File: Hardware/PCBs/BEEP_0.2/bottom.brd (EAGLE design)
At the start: 85 x 73 mm, 53 parts, among them IC1 74HCT00D, Q1 DMN2075U, Q2 IRLML2244, Q5 IRLML2244, Q6 IRLML2244, Q8 IRLML2244, U1 LM239AMDREP, U2 ATTINY10-TSHR

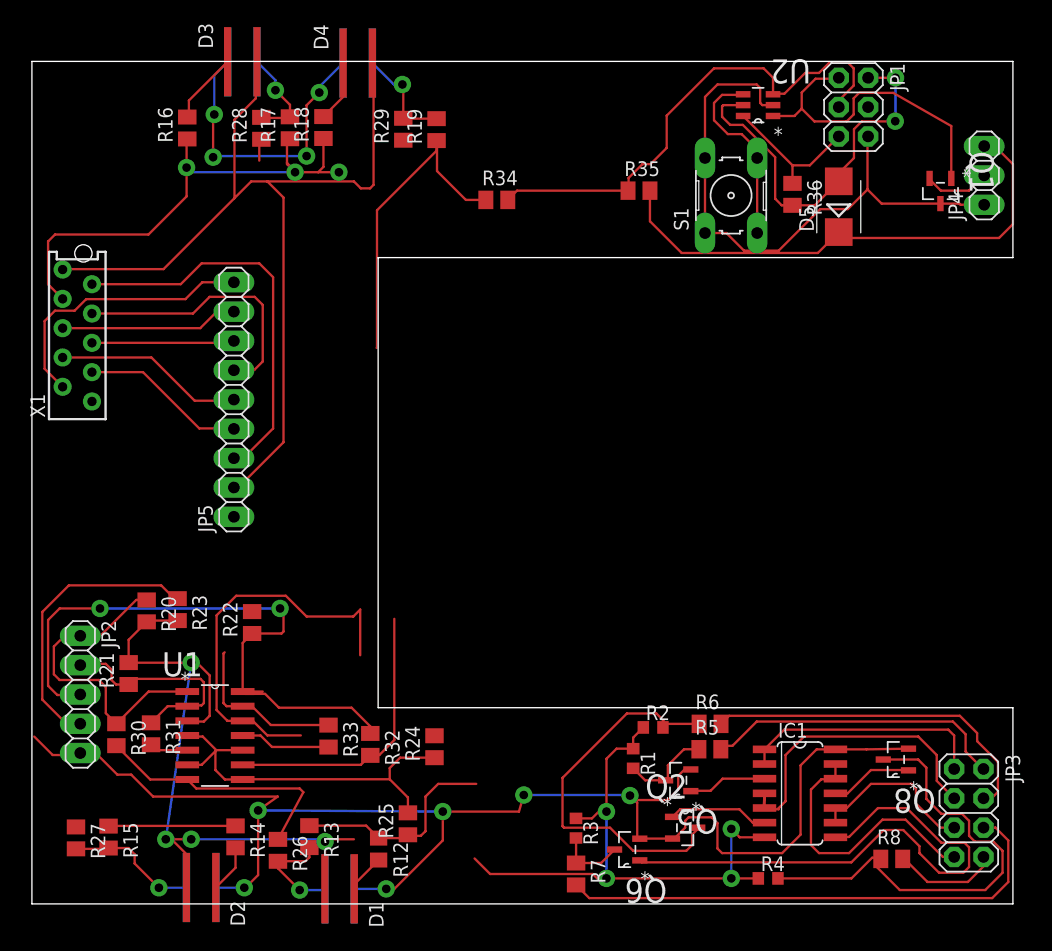
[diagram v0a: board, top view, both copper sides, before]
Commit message: continue work on bottom pcbs
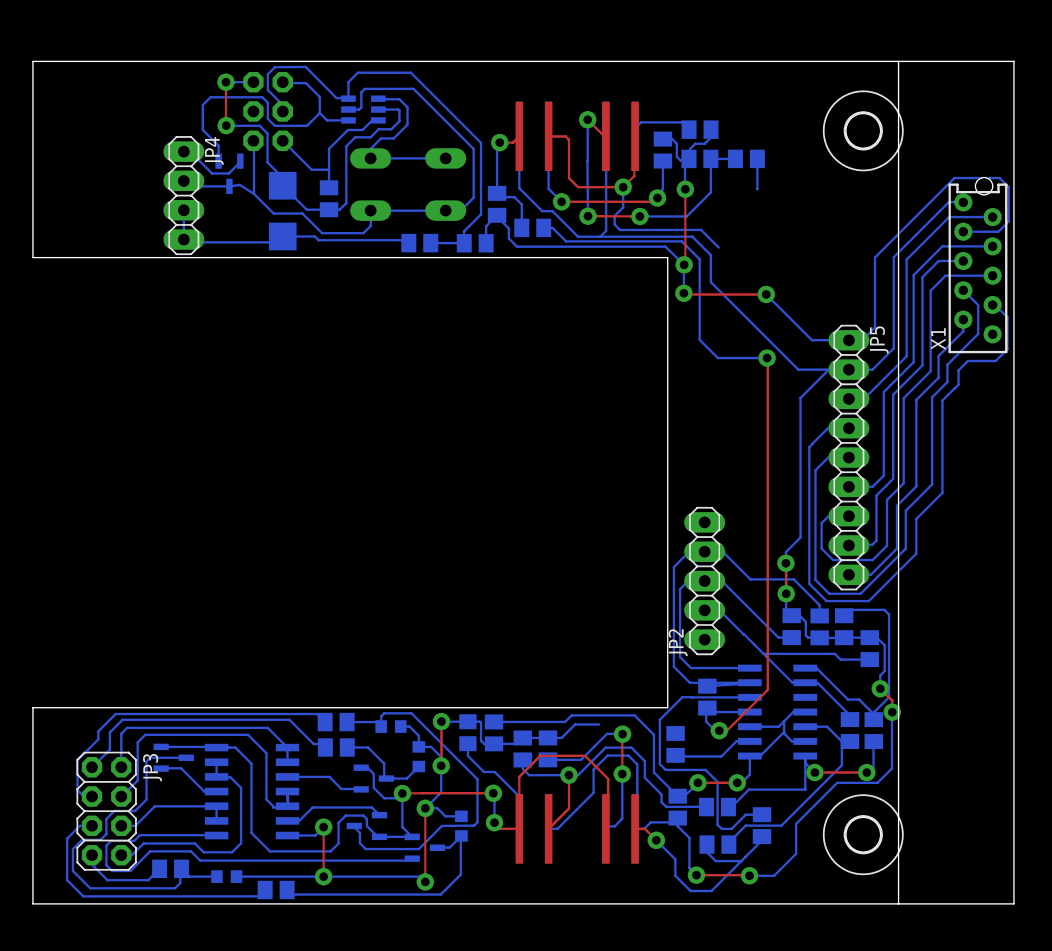
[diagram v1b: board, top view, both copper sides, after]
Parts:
- added U$1, U$2: (no value), holes:3,0
- JP4: device pinhead:1X03 -> pinhead:1X04
- moved X1 78.3 mm to (82.0, 55.1)
- moved JP3 74.7 mm to (6.48, 8.03)
- moved JP4 69.4 mm to (13.2, 61.4), turned to 270 degrees
- moved R30 65.6 mm to (72.9, 15.0), flipped to the bottom
- moved R21 64.3 mm to (72.6, 22.1), flipped to the bottom
- moved Q8 62.6 mm to (12.3, 12.7), flipped to the bottom
- moved R8 62.5 mm to (12.0, 3.04), flipped to the bottom
- moved Q1 61.6 mm to (17.1, 63.3), flipped to the bottom
- moved R31 60.6 mm to (70.9, 15.0), flipped to the bottom
- moved R20 60.5 mm to (70.4, 24.0), flipped to the bottom
- moved R15 56.6 mm to (63.3, 6.78), flipped to the bottom
- moved R23 55.7 mm to (68.3, 24.0), flipped to the bottom
- moved R27 55.6 mm to (59.4, 5.14), flipped to the bottom, turned to 0 degrees
- moved JP2 55.0 mm to (58.3, 28.0), turned to 90 degrees
- moved JP5 53.5 mm to (70.8, 38.7), turned to 270 degrees
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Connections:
- net +7V: now also JP4.4
- net BATT_GND: now also JP4.2; no longer JP4.1
- net PWM_IN1: now also JP3.2; no longer JP3.1
- net PWM_IN2: now also JP3.4; no longer JP3.3
- net PWM_IN3: now also JP3.6; no longer JP3.5
- net PWM_IN4: now also JP3.8; no longer JP3.7
- net PWM_OUT1: now also JP3.1; no longer JP3.2
- net PWM_OUT2: now also JP3.3; no longer JP3.4
- net PWM_OUT3: now also JP3.5; no longer JP3.6
- net PWM_OUT4: now also JP3.7; no longer JP3.8
- net SWITCHED_GND: now also JP4.1; no longer JP4.2
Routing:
- net N$49: track 7.85 -> 69.1 mm, vias 0 -> 2
- net +5V: track 153.8 -> 103.0 mm, vias 10 -> 4
- net COLOR_DIODE_2: track 14.3 -> 54.5 mm
- net COLOR_DIODE_1: track 16.4 -> 48.3 mm
- net ENC_R1: track 54.3 -> 24.8 mm, vias 2 -> 0
- net COLOR_SENSOR_3: track 12.4 -> 41.0 mm
- net +3V3: track 144.8 -> 167.8 mm, vias 4 -> 6
- net +7V: track 45.0 -> 22.6 mm
- net PWM_OUT3: track 44.7 -> 24.2 mm
- net ENC_L1_RAW: track 9.21 -> 26.7 mm
- net ENC_R1_RAW: track 9.66 -> 27.1 mm, vias 1 -> 3
- net N$47: track 26.5 -> 9.64 mm
- net N$14: track 5.98 -> 21.9 mm
- net N$45: track 3.33 -> 19.2 mm
- net COLOR_SENSOR_2: track 15.4 -> 31.2 mm
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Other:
- outline, holes or cut-outs redrawn
